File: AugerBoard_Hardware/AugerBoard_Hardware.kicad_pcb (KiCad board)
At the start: 2 copper layers, 44 parts, among them J1 RJ45_LED_Shielded, J2 Conn_01x04_MountingPin, Q1 BSS138, Q2 BSS138, Q3 BSS138, SW1 SW_SPDT, SW2 SW_Push, SW3 SW_Push, SW4 SW_Push, U1 Teensy4.1_DEV-16771, U2 OKI-78SR-5_1.5-W36H-C

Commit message: Good first pass hai
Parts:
- moved J2 43.3 mm to (173.2, 135.4)
- moved D6 16.9 mm to (163.0, 95.6), turned to 180 degrees
- moved R6 16.9 mm to (163.0, 98.2), turned to 180 degrees
- moved SW4 16.9 mm to (160.1, 91.4)
- moved Q3 16.9 mm to (157.6, 97.2)
- moved D1 8.02 mm to (103.6, 104.1), turned to 180 degrees
- moved R5 6.70 mm to (99.8, 96.3), turned to 0 degrees
- moved Q2 6.12 mm to (157.5, 79.9)
- moved SW3 6.10 mm to (160.0, 74.7)
- moved R2 6.10 mm to (162.9, 81.5), turned to 180 degrees
- moved D5 5.99 mm to (162.8, 79.0), turned to 180 degrees
- moved D2 3.67 mm to (103.6, 100.3), turned to 180 degrees
- moved R3 3.31 mm to (99.7, 104.1), turned to 0 degrees
- moved SW2 3.15 mm to (146.8, 74.7)
- moved Q1 3.15 mm to (144.0, 80.0)
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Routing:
- net +3.3V: track 0.00 -> 196.8 mm, vias 0 -> 7
- net PWM1: track 0.00 -> 107.9 mm, vias 0 -> 3
- net PWM3: track 0.00 -> 85.5 mm, vias 0 -> 4
- net Temp: track 0.00 -> 85.4 mm, vias 0 -> 1
- net PWM2: track 0.00 -> 79.0 mm, vias 0 -> 3
- net GND: track 0.00 -> 72.5 mm, vias 0 -> 1
- net IN_B3: track 0.00 -> 63.7 mm, vias 0 -> 2
- net LimitSwitch2: track 0.00 -> 60.8 mm, vias 0 -> 2
- net LED: track 0.00 -> 58.9 mm, vias 0 -> 1
- net Humidity: track 0.00 -> 51.1 mm
- net LimitSwitch1: track 0.00 -> 51.0 mm, vias 0 -> 2
- net IN_A3: track 0.00 -> 50.8 mm
- net IN_A1: track 0.00 -> 50.6 mm, vias 0 -> 1
- net Dir_Switch: track 0.00 -> 47.2 mm, vias 0 -> 2
- net T+: track 0.00 -> 43.6 mm, vias 0 -> 1
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- removed copper zone on B.Cu, net +12V
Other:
- board outline added: 103.1 x 87.6 mm

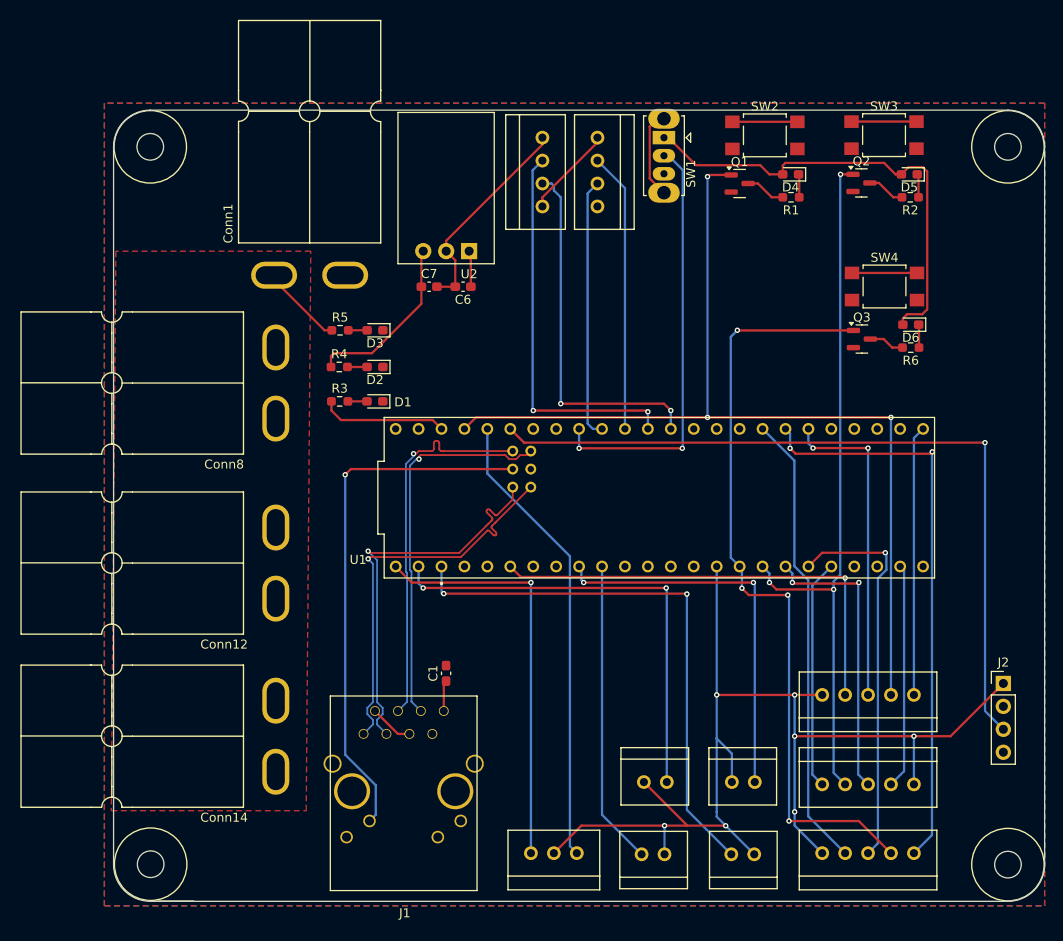
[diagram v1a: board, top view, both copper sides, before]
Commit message: Layout made smaller h
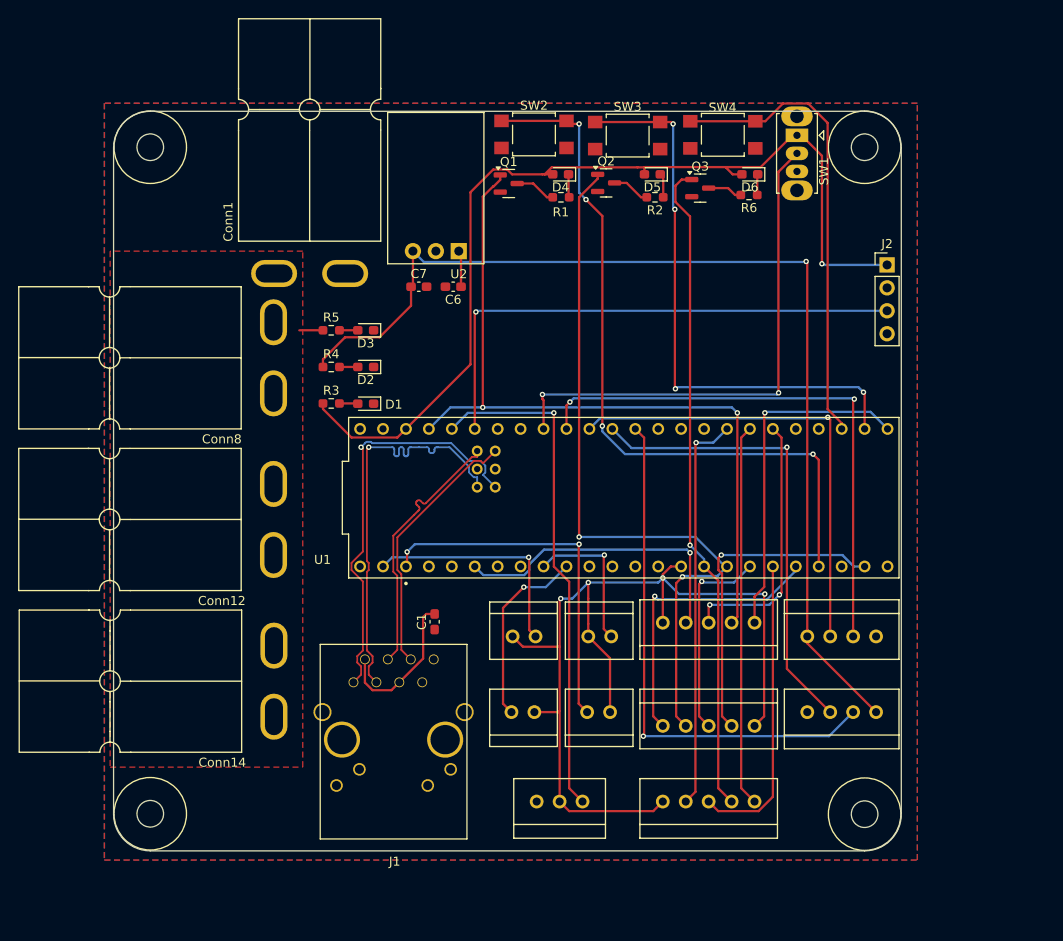
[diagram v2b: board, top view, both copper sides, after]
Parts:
- moved Conn2 67.1 mm to (159.1, 138.6), turned to 180 degrees
- moved Conn3 59.9 mm to (151.5, 130.2), turned to 0 degrees
- moved J2 48.1 mm to (160.4, 89.0)
- moved D5 28.5 mm to (134.4, 79.0)
- moved SW3 28.4 mm to (131.6, 74.7)
- moved R2 28.3 mm to (134.6, 81.5)
- moved Q2 28.3 mm to (129.2, 79.9)
- moved Q1 25.6 mm to (118.4, 80.0)
- moved SW2 25.6 mm to (121.2, 74.6)
- moved R1 25.5 mm to (124.2, 81.5)
- moved D4 25.5 mm to (124.2, 79.0)
- moved R6 24.6 mm to (145.1, 81.3)
- moved SW4 24.6 mm to (142.2, 74.6)
- moved Q3 24.5 mm to (139.7, 80.5)
- moved D6 24.4 mm to (145.1, 79.0)
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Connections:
- Conn1 pad 4: +12V -> (no net)
- Conn12 pad 4: +12V -> (no net)
- Conn14 pad : +12V -> (no net)
- Conn8 pad 4: +12V -> (no net)
- U1 pad 41: SEL3 -> unconnected-(U1-A17-Pad41)
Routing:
- net +5V: track 29.7 -> 116.4 mm, vias 0 -> 1
- net SW1: track 7.20 -> 80.9 mm, vias 0 -> 4
- net GND: track 72.5 -> 0.00 mm, vias 1 -> 0
- net LED: track 58.9 -> 0.00 mm, vias 1 -> 0
- net SW2: track 7.20 -> 63.4 mm, vias 0 -> 4
- net SW3: track 7.20 -> 51.4 mm
- net Encoder_2b: track 28.9 -> 61.2 mm, vias 0 -> 2
- net Temp: track 85.4 -> 58.6 mm
- net LimitSwitch3: track 42.9 -> 16.6 mm, vias 2 -> 1
- net LimitSwitch1: track 51.0 -> 25.6 mm, vias 2 -> 1
- net PWM1: track 107.9 -> 85.5 mm, vias 3 -> 2
- net IN_B3: track 63.7 -> 42.3 mm, vias 2 -> 0
- net LimitSwitch2: track 60.8 -> 40.1 mm
- net Encoder_2a: track 31.0 -> 51.3 mm, vias 0 -> 1
- net Encoder_1a: track 40.4 -> 58.8 mm, vias 2 -> 1
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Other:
- board size 103.1 x 87.6 mm -> 87.2 x 81.9 mm
